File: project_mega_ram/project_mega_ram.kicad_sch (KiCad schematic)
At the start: 28 parts, among them U1 74LS670, U10 74LS02, U11 74LS139, U12 CS18LV10245, U2 CS18LV10245, U3 74LS670, U4 74LS157, U5 74LS157, U6 74LS08, U7 74LS32, U8 74LS74, U9 74LS32

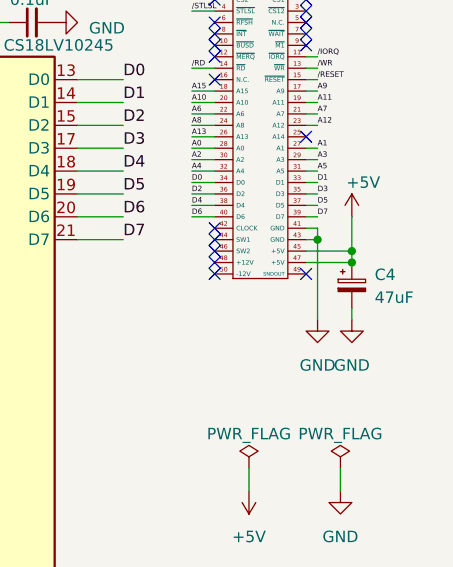
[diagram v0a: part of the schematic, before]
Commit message: modified PCB : Signed-off-by: ykp74 <ykp7409@gmail.com>
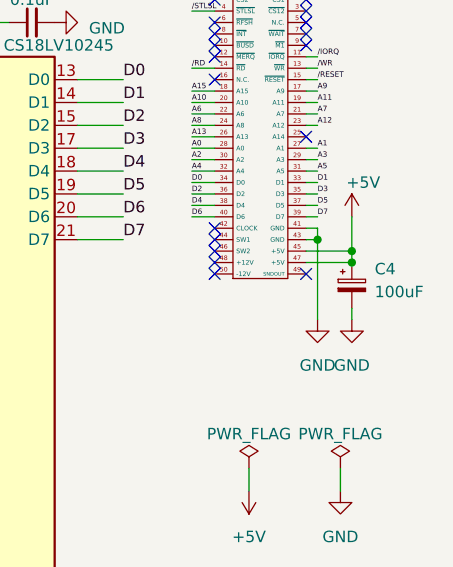
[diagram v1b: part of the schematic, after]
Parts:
- C4: value 47uF -> 100uF
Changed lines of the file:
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@@
 		(fields_autoplaced yes)
 		(property "Reference" "C4"
-			(at 283.21 50.8889 0)
+			(at 283.21 50.2538 0)
 			(show_name no)
 			(do_not_autoplace no)
@@
 			)
 		)
-		(property "Value" "47uF"
-			(at 283.21 53.4289 0)
+		(property "Value" "100uF"
+			(at 283.21 52.7938 0)
 			(show_name no)
 			(do_not_autoplace no)
